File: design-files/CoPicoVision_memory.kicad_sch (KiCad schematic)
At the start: 9 parts, among them U103 74ACT05, U201 GAL22V10, U202 GAL22V10, U203 AT28C64, U204 AS6C6264

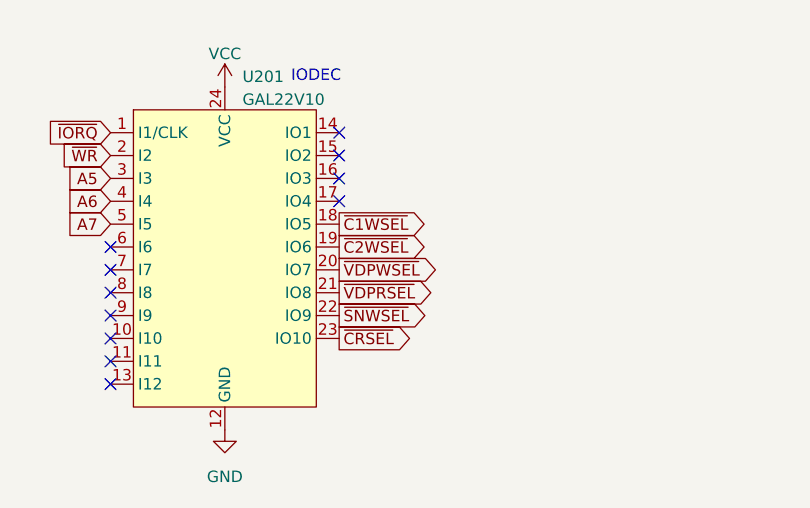
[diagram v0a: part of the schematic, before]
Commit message: Added video circuit.
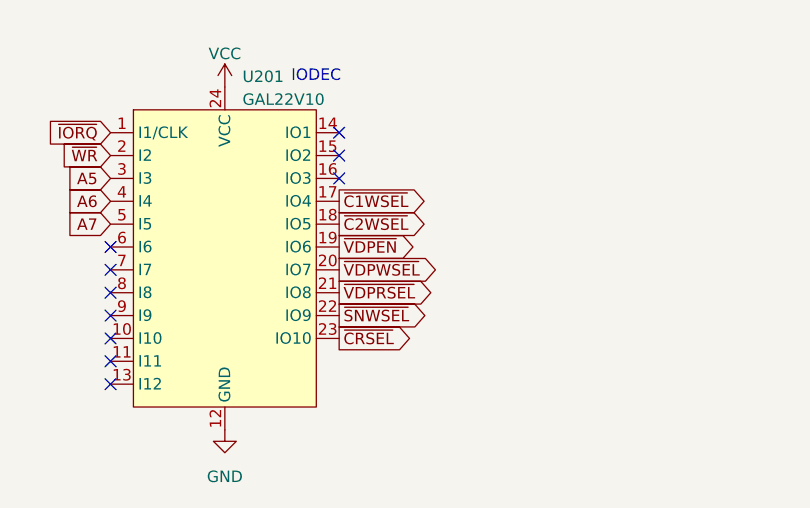
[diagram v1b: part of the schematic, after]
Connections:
- net ~{C1WSEL}: now also U201.17 (IO4); no longer U201.18 (IO5)
- net ~{C2WSEL}: now also U201.18 (IO5); no longer U201.19 (IO6)
- new net ~{VDPEN}: U201.19 (IO6)
- no-connect marks 19 -> 18

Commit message: Get footprints on everything.
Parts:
- C201, C202, C203, C204: footprint (none) -> Capacitor_THT:C_Disc_D3.8mm_W2.6mm_P2.50mm
- U103: footprint (none) -> Package_DIP:DIP-14_W7.62mm_Socket
- U204: footprint Package_DIP:DIP-28_W15.24mm -> Package_DIP:DIP-28_W15.24mm_Socket
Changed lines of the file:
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@@
       (effects (font (size 1.27 1.27)) (justify left))
     )
-    (property "Footprint" "" (at 110.871 158.496 0)
+    (property "Footprint" "Capacitor_THT:C_Disc_D3.8mm_W2.6mm_P2.50mm" (at 110.871 158.496 0)
       (effects (font (size 1.27 1.27)) hide)
     )
@@
       (effects (font (size 1.27 1.27)) (justify left))
     )
-    (property "Footprint" "" (at 87.884 158.496 0)
+    (property "Footprint" "Capacitor_THT:C_Disc_D3.8mm_W2.6mm_P2.50mm" (at 87.884 158.496 0)
       (effects (font (size 1.27 1.27)) hide)
     )
@@
       (effects (font (size 1.27 1.27)) (justify left))
     )
-    (property "Footprint" "" (at 76.454 158.496 0)
+    (property "Footprint" "Capacitor_THT:C_Disc_D3.8mm_W2.6mm_P2.50mm" (at 76.454 158.496 0)
       (effects (font (size 1.27 1.27)) hide)
     )
@@
       (effects (font (size 1.27 1.27)) (justify left))
     )
-    (property "Footprint" "" (at 99.441 158.496 0)
+    (property "Footprint" "Capacitor_THT:C_Disc_D3.8mm_W2.6mm_P2.50mm" (at 99.441 158.496 0)
       (effects (font (size 1.27 1.27)) hide)
     )
@@
       (effects (font (size 1.27 1.27)) (justify left))
     )
-    (property "Footprint" "Package_DIP:DIP-28_W15.24mm" (at 201.295 127 0)
+    (property "Footprint" "Package_DIP:DIP-28_W15.24mm_Socket" (at 201.295 127 0)
       (effects (font (size 1.27 1.27)) hide)
     )
@@
       (effects (font (size 1.27 1.27)))
     )
-    (property "Footprint" "" (at 143.129 106.299 0)
-      (effects (font (size 1.27 1.27)) hide)
-    )
+    (property "Footprint" "Package_DIP:DIP-14_W7.62mm_Socket" (at 143.129 106.299 0)
+      (effects (font (size 1.27 1.27)) hide)
+    )

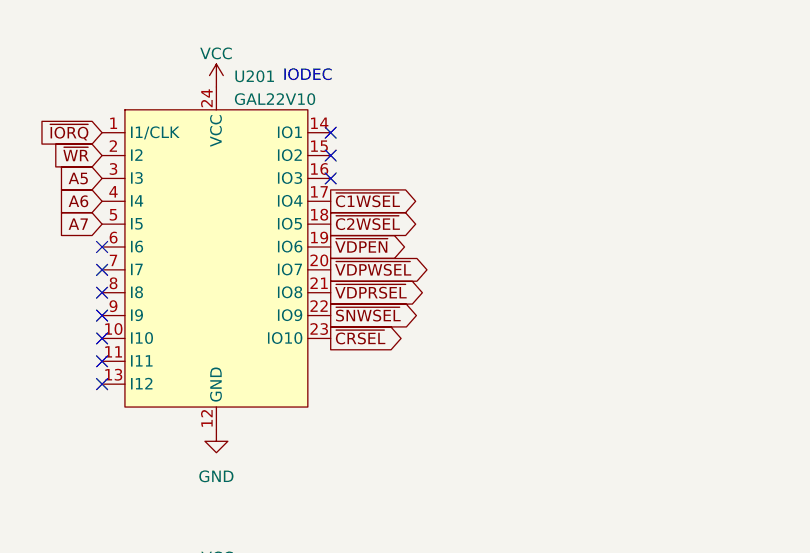
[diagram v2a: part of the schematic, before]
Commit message: Shuffle IODEC outputs to make layout easier.
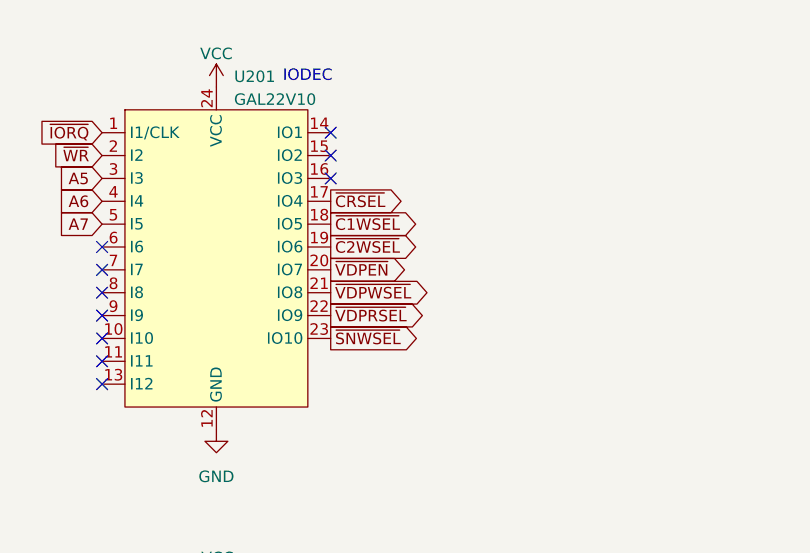
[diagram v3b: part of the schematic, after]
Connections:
- net ~{C1WSEL}: now also U201.18 (IO5); no longer U201.17 (IO4)
- net ~{C2WSEL}: now also U201.19 (IO6); no longer U201.18 (IO5)
- net ~{CRSEL}: now also U201.17 (IO4); no longer U201.23 (IO10)
- net ~{SNWSEL}: now also U201.23 (IO10); no longer U201.22 (IO9)
- net ~{VDPEN}: now also U201.20 (IO7); no longer U201.19 (IO6)
- net ~{VDPRSEL}: now also U201.22 (IO9); no longer U201.21 (IO8)
- net ~{VDPWSEL}: now also U201.21 (IO8); no longer U201.20 (IO7)
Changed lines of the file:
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@@
     )
   )
-  (global_label "~{VDPWSEL}" (shape output) (at 121.158 62.992 0) (fields_autoplaced)
-    (effects (font (size 1.27 1.27)) (justify left))
-    (property "Intersheetrefs" "${INTERSHEET_REFS}" (at 132.5304 62.992 0)
+  (global_label "~{VDPWSEL}" (shape output) (at 121.158 65.532 0) (fields_autoplaced)
+    (effects (font (size 1.27 1.27)) (justify left))
+    (property "Intersheetrefs" "${INTERSHEET_REFS}" (at 132.5304 65.532 0)
       (effects (font (size 1.27 1.27)) (justify left) hide)
     )
@@
     )
   )
-  (global_label "~{C1WSEL}" (shape output) (at 121.158 55.372 0) (fields_autoplaced)
-    (effects (font (size 1.27 1.27)) (justify left))
-    (property "Intersheetrefs" "${INTERSHEET_REFS}" (at 131.3813 55.372 0)
+  (global_label "~{C1WSEL}" (shape output) (at 121.158 57.912 0) (fields_autoplaced)
+    (effects (font (size 1.27 1.27)) (justify left))
+    (property "Intersheetrefs" "${INTERSHEET_REFS}" (at 131.3813 57.912 0)
       (effects (font (size 1.27 1.27)) (justify left) hide)
     )
@@
     )
   )
-  (global_label "~{CRSEL}" (shape output) (at 121.158 70.612 0) (fields_autoplaced)
-    (effects (font (size 1.27 1.27)) (justify left))
-    (property "Intersheetrefs" "${INTERSHEET_REFS}" (at 129.9904 70.612 0)
+  (global_label "~{CRSEL}" (shape output) (at 121.158 55.372 0) (fields_autoplaced)
+    (effects (font (size 1.27 1.27)) (justify left))
+    (property "Intersheetrefs" "${INTERSHEET_REFS}" (at 129.9904 55.372 0)
       (effects (font (size 1.27 1.27)) (justify left) hide)
     )
@@
     )
   )
-  (global_label "~{VDPEN}" (shape output) (at 121.158 60.452 0) (fields_autoplaced)
-    (effects (font (size 1.27 1.27)) (justify left))
-    (property "Intersheetrefs" "${INTERSHEET_REFS}" (at 130.1719 60.452 0)
+  (global_label "~{VDPEN}" (shape output) (at 121.158 62.992 0) (fields_autoplaced)
+    (effects (font (size 1.27 1.27)) (justify left))
+    (property "Intersheetrefs" "${INTERSHEET_REFS}" (at 130.1719 62.992 0)
       (effects (font (size 1.27 1.27)) (justify left) hide)
     )
@@
     )
   )
-  (global_label "~{SNWSEL}" (shape output) (at 121.158 68.072 0) (fields_autoplaced)
-    (effects (font (size 1.27 1.27)) (justify left))
-    (property "Intersheetrefs" "${INTERSHEET_REFS}" (at 131.4418 68.072 0)
+  (global_label "~{SNWSEL}" (shape output) (at 121.158 70.612 0) (fields_autoplaced)
+    (effects (font (size 1.27 1.27)) (justify left))
+    (property "Intersheetrefs" "${INTERSHEET_REFS}" (at 131.4418 70.612 0)
       (effects (font (size 1.27 1.27)) (justify left) hide)
     )
@@
     )
   )
-  (global_label "~{C2WSEL}" (shape output) (at 121.158 57.912 0) (fields_autoplaced)
-    (effects (font (size 1.27 1.27)) (justify left))
-    (property "Intersheetrefs" "${INTERSHEET_REFS}" (at 131.3813 57.912 0)
+  (global_label "~{C2WSEL}" (shape output) (at 121.158 60.452 0) (fields_autoplaced)
+    (effects (font (size 1.27 1.27)) (justify left))
+    (property "Intersheetrefs" "${INTERSHEET_REFS}" (at 131.3813 60.452 0)
       (effects (font (size 1.27 1.27)) (justify left) hide)
     )
@@
     )
   )
-  (global_label "~{VDPRSEL}" (shape output) (at 121.158 65.532 0) (fields_autoplaced)
-    (effects (font (size 1.27 1.27)) (justify left))
-    (property "Intersheetrefs" "${INTERSHEET_REFS}" (at 132.349 65.532 0)
-      (effects (font (size 1.27 1.27)) (justify left) hide)
-    )
+  (global_label "~{VDPRSEL}" (shape output) (at 121.158 68.072 0) (fields_autoplaced)
+    (effects (font (size 1.27 1.27)) (justify left))
+    (property "Intersheetrefs" "${INTERSHEET_REFS}" (at 132.349 68.072 0)
+      (effects (font (size 1.27 1.27)) (justify left) hide)
+    )

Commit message: BoM.
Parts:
- C201, C202, C203, C204: Mouser (none) -> 81-RCER71E104K0A2H3B
- U103: Mouser (none) -> 595-CD74ACT05EE4
- U201, U202: Mouser (none) -> 556-AF22V10C15PU
- U203: Mouser (none) -> 556-AT28C64B15PU
- U204: Mouser (none) -> 913-AS6C6264-55PCN
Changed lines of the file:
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@@
+      (effects (font (size 1.27 1.27)) hide)
+    )
+    (property "Mouser" "81-RCER71E104K0A2H3B" (at 110.871 158.496 0)
       (effects (font (size 1.27 1.27)) hide)
     )
@@
       (effects (font (size 1.27 1.27)) hide)
     )
+    (property "Mouser" "81-RCER71E104K0A2H3B" (at 87.884 158.496 0)
+      (effects (font (size 1.27 1.27)) hide)
+    )
     (pin "1")
     (pin "2")
@@
       (effects (font (size 1.27 1.27)) hide)
     )
+    (property "Mouser" "81-RCER71E104K0A2H3B" (at 76.454 158.496 0)
+      (effects (font (size 1.27 1.27)) hide)
+    )
     (pin "1")
     (pin "2")
@@
     )
     (property "Datasheet" "~" (at 99.441 158.496 0)
+      (effects (font (size 1.27 1.27)) hide)
+    )
+    (property "Mouser" "81-RCER71E104K0A2H3B" (at 99.441 158.496 0)
       (effects (font (size 1.27 1.27)) hide)
     )
@@
     )
     (property "Datasheet" "" (at 108.585 117.729 0)
+      (effects (font (size 1.27 1.27)) hide)
+    )
+    (property "Mouser" "556-AF22V10C15PU" (at 108.585 117.729 0)
       (effects (font (size 1.27 1.27)) hide)
     )
@@
     )
     (property "Datasheet" "https://www.mouser.com/datasheet/2/12/Alliance%20Memory_64K_AS6C6264v2.0July2017-1144693.pdf" (at 201.295 127 0)
+      (effects (font (size 1.27 1.27)) hide)
+    )
+    (property "Mouser" "913-AS6C6264-55PCN" (at 201.295 119.38 0)
       (effects (font (size 1.27 1.27)) hide)
     )
@@
       (effects (font (size 1.27 1.27)) hide)
     )
+    (property "Mouser" "556-AT28C64B15PU" (at 200.279 64.135 0)
+      (effects (font (size 1.27 1.27)) hide)
+    )
     (pin "10")
     (pin "11")
@@
       (effects (font (size 1.27 1.27)) hide)
     )
+    (property "Mouser" "556-AF22V10C15PU" (at 108.458 61.722 0)
+      (effects (font (size 1.27 1.27)) hide)
+    )
     (pin "1")
     (pin "10")
@@
       (effects (font (size 1.27 1.27)) hide)
     )
+    (property "Mouser" "595-CD74ACT05EE4" (at 143.129 106.299 0)
+      (effects (font (size 1.27 1.27)) hide)
+    )
